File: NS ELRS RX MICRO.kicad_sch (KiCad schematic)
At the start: 39 parts, among them J1 Conn_Coaxial, J2 Conn_Coaxial, U1 ESP32-C3, U2 SX1280IMLTRT, U3 SE2431L-R, U4 LP5912-3.3DRV, Y1 52MHz, 8pF, Y2 40MHz, 8pF

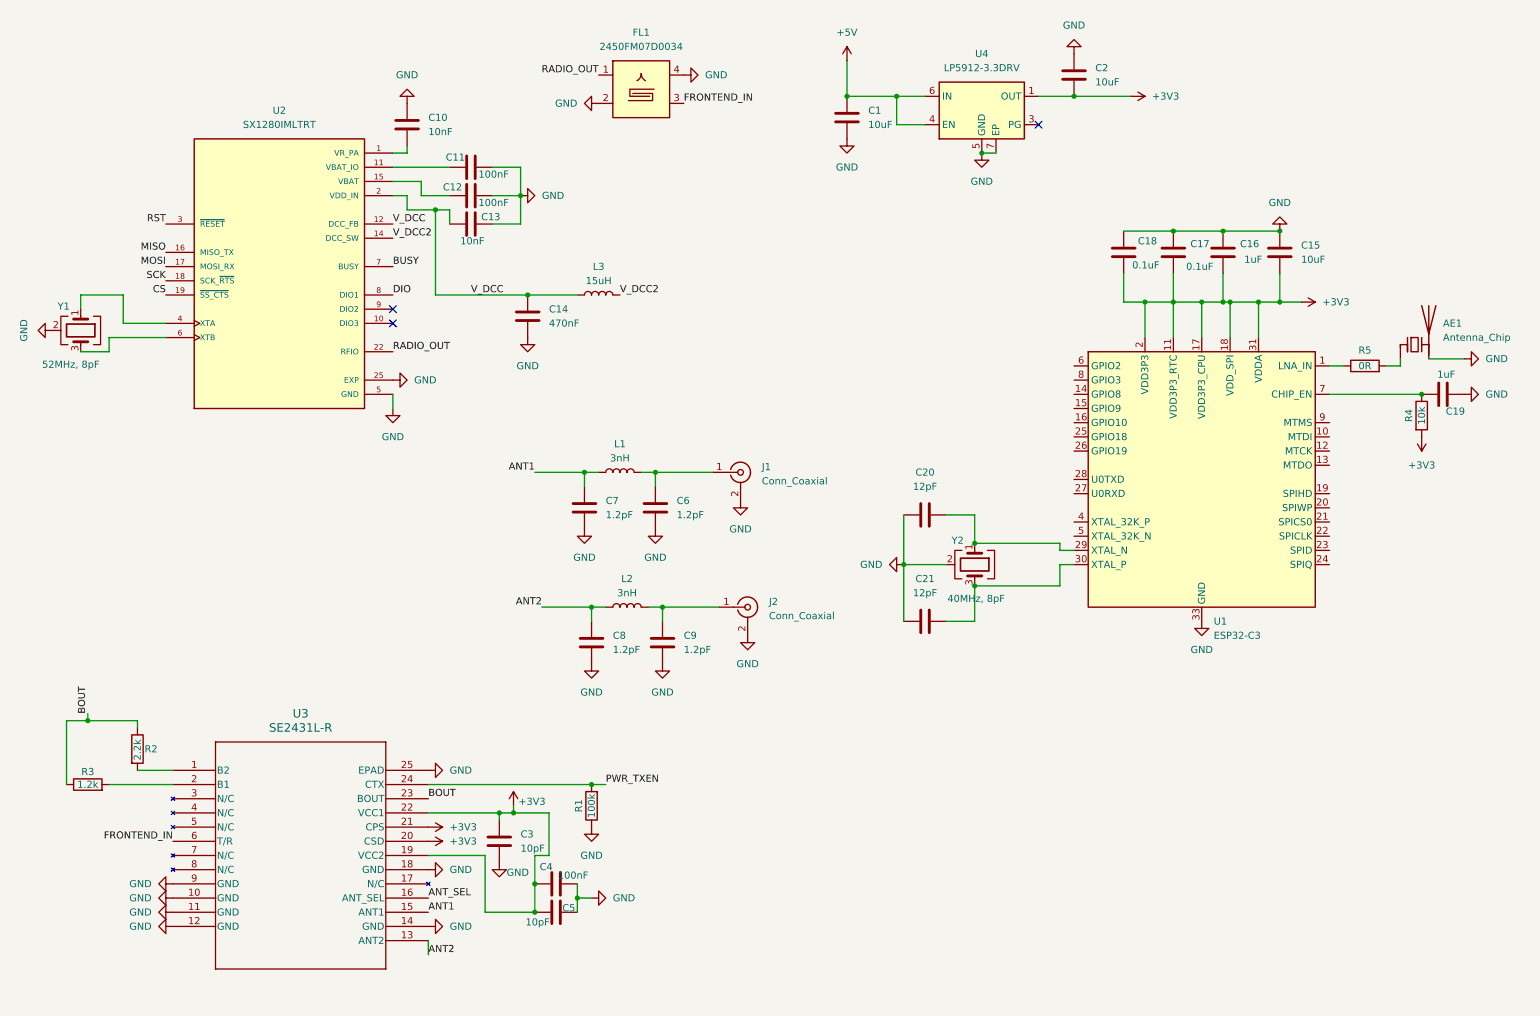
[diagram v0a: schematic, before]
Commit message: completed schematic
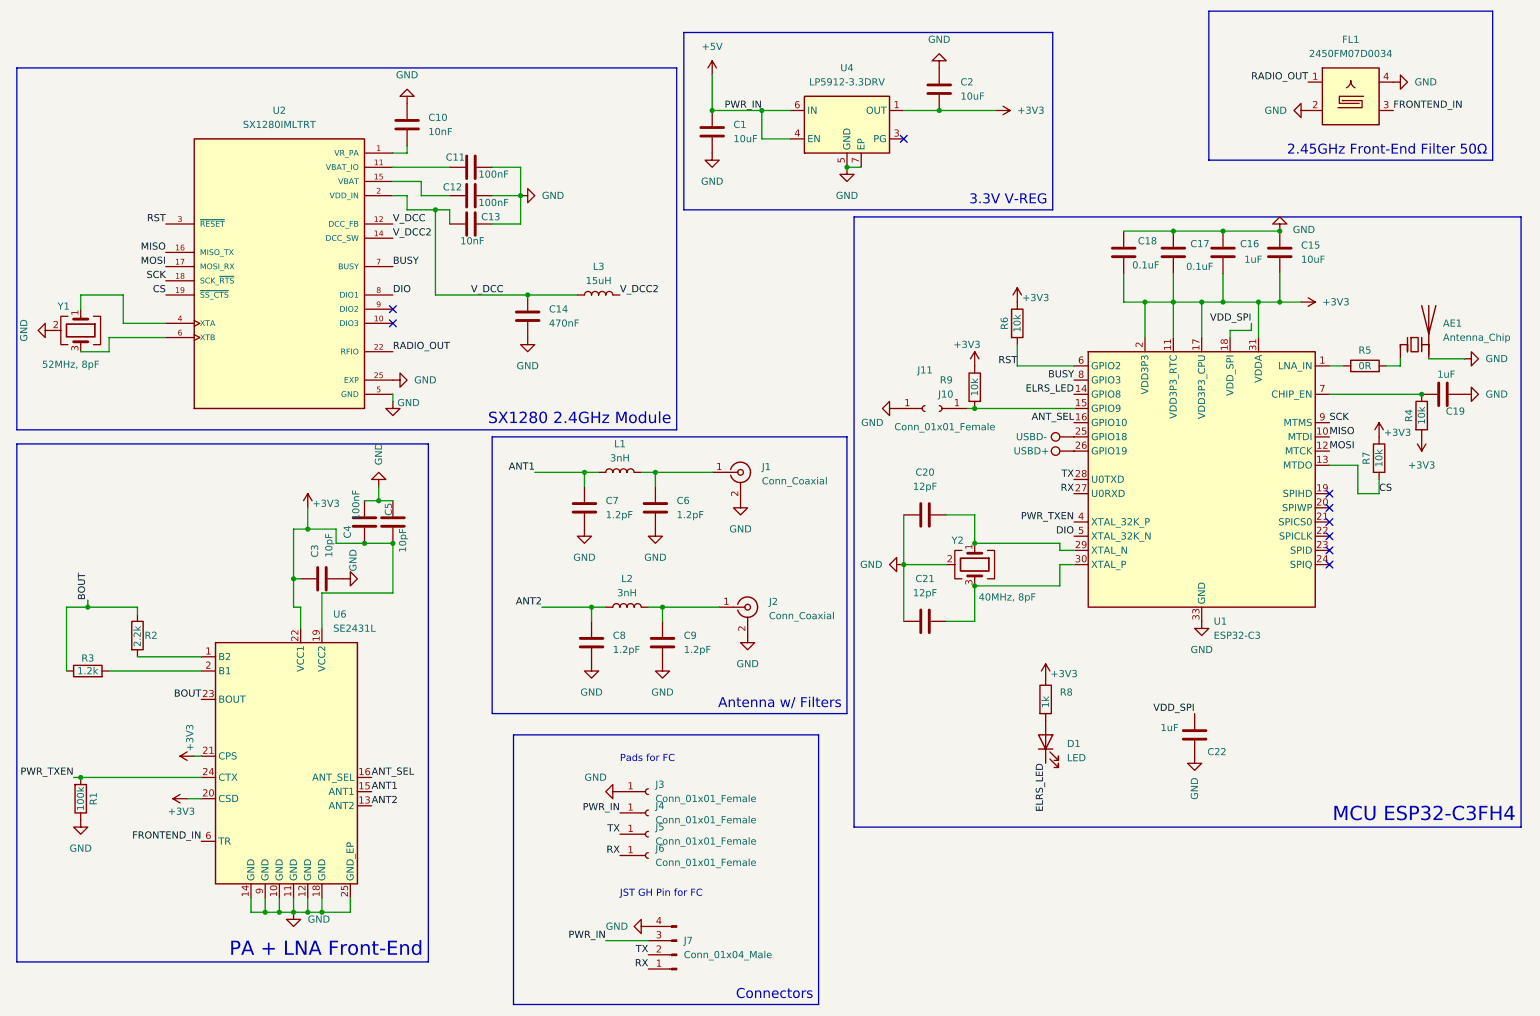
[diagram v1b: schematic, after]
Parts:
- removed U3: SE2431L-R, SE2431L_SKY, symbol 2026-10-20_12-47-49:SE2431L-R
- added C22: 1uF, Package_SON:WSON-6-1EP_2x2mm_P0.65mm_EP1x1.6mm_ThermalVias, symbol Device:C
- added D1: LED, symbol Device:LED
- added J10, J11: Conn_01x01_Female, TestPoint:TestPoint_Pad_1.0x1.0mm, symbol Connector:Conn_01x01_Female
- added J3, J4, J5, J6: Conn_01x01_Female, TestPoint:TestPoint_Pad_2.5x2.5mm, symbol Connector:Conn_01x01_Female
- added J7: Conn_01x04_Male, Connector_JST:JST_GH_SM04B-GHS-TB_1x04-1MP_P1.25mm_Horizontal, symbol Connector:Conn_01x04_Male
- added R6, R7: 10k, symbol Device:R
- added R8: 1k, symbol Device:R
- added R9: 10k, Resistor_SMD:R_0402_1005Metric, symbol Device:R
- added TP1: USBD-, Package_DIP:DIP-16_W7.62mm, symbol Connector:TestPoint
- added TP2: USBD+, Package_DIP:DIP-16_W7.62mm, symbol Connector:TestPoint
- added U6: SE2431L, Package_DFN_QFN:QFN-24-1EP_3x4mm_P0.4mm_EP1.65x2.65mm, symbol Anyleaf Shared:SE2431L
- AE1: footprint Oscillator:Oscillator_SMD_SeikoEpson_SG210-4Pin_2.5x2.0mm -> RF_Antenna:Johanson_2450AT18x100
- FL1: footprint Filter:Filter_1109-5_1.1x0.9mm -> 2450FM07D0034:2450FM07D0034
- J1, J2: footprint Package_SON:WSON-6-1EP_2x2mm_P0.65mm_EP1x1.6mm_ThermalVias -> Connector_Coaxial:U.FL_Hirose_U.FL-R-SMT-1_Vertical
- U4: footprint Package_SON:WSON-6-1EP_2x2mm_P0.65mm_EP1x1.6mm_ThermalVias -> Package_TO_SOT_SMD:TSOT-23-5
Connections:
- net +3V3: now also R6.1, R7.1, R8.1, R9.1, U6.19 (VCC2), U6.20 (CSD), U6.21 (CPS), U6.22 (VCC1); no longer U1.18 (VDD_SPI)
- net +5V: now also J4.1 (Pin_1), J7.3 (Pin_3)
- net ANT1: now also U6.15 (ANT1)
- net ANT2: now also U6.13 (ANT2)
- net ANT_SEL: now also U1.16 (GPIO10), U6.16 (ANT_SEL)
- net BOUT: now also U6.23 (BOUT)
- net BUSY: now also U1.8 (GPIO3)
- net CS: now also U1.13 (MTDO), R7.2
- net DIO: now also U1.5 (XTAL_32K_N)
- net FRONTEND_IN: now also U6.6 (TR)
- net GND: now also C22.2, J11.1 (Pin_1), J3.1 (Pin_1), J7.4 (Pin_4), U6.10 (GND), U6.11 (GND), U6.12 (GND), U6.14 (GND), U6.18 (GND), U6.25 (GND_EP), U6.9 (GND)
- net MISO: now also U1.10 (MTDI)
- net MOSI: now also U1.12 (MTCK)
- net PWR_TXEN: now also U1.4 (XTAL_32K_P), U6.24 (CTX)
- net RST: now also U1.6 (GPIO2), R6.2
- net SCK: now also U1.9 (MTMS)
- net at R2.2: now also U6.1 (B2)
- net at R3.2: now also U6.2 (B1)
- net ELRS_LED: now reaches U1.14 (GPIO8)
- net ELRS_LED: now also D1.1 (K)
- net at U1.15 (GPIO9): now also J10.1 (Pin_1), R9.2
- net at U1.25 (GPIO18): now also TP1.1
- net at U1.26 (GPIO19): now also TP2.1
- net RX: now reaches U1.27 (U0RXD)
- net RX: now also J6.1 (Pin_1), J7.1 (Pin_1)
- net TX: now reaches U1.28 (U0TXD)
- net TX: now also J5.1 (Pin_1), J7.2 (Pin_2)
- new net: D1.2 (A), R8.2
- new net VDD_SPI: C22.1, U1.18 (VDD_SPI)
- no-connect marks 3 -> 9
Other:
- note added: "JST GH Pin for FC"
- note added: "Pads for FC"
- moved on the sheet: C1, C2, C3, C4, C5, FL1, R1, R2, R3, U4
